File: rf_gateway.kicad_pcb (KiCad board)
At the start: 2 copper layers, 48.2 x 23.3 mm, 7 parts, among them J101 PJ-202A, J102 Conn_01x03_Female, J103 Conn_01x05_Male, U101 ESP32-WROOM-32

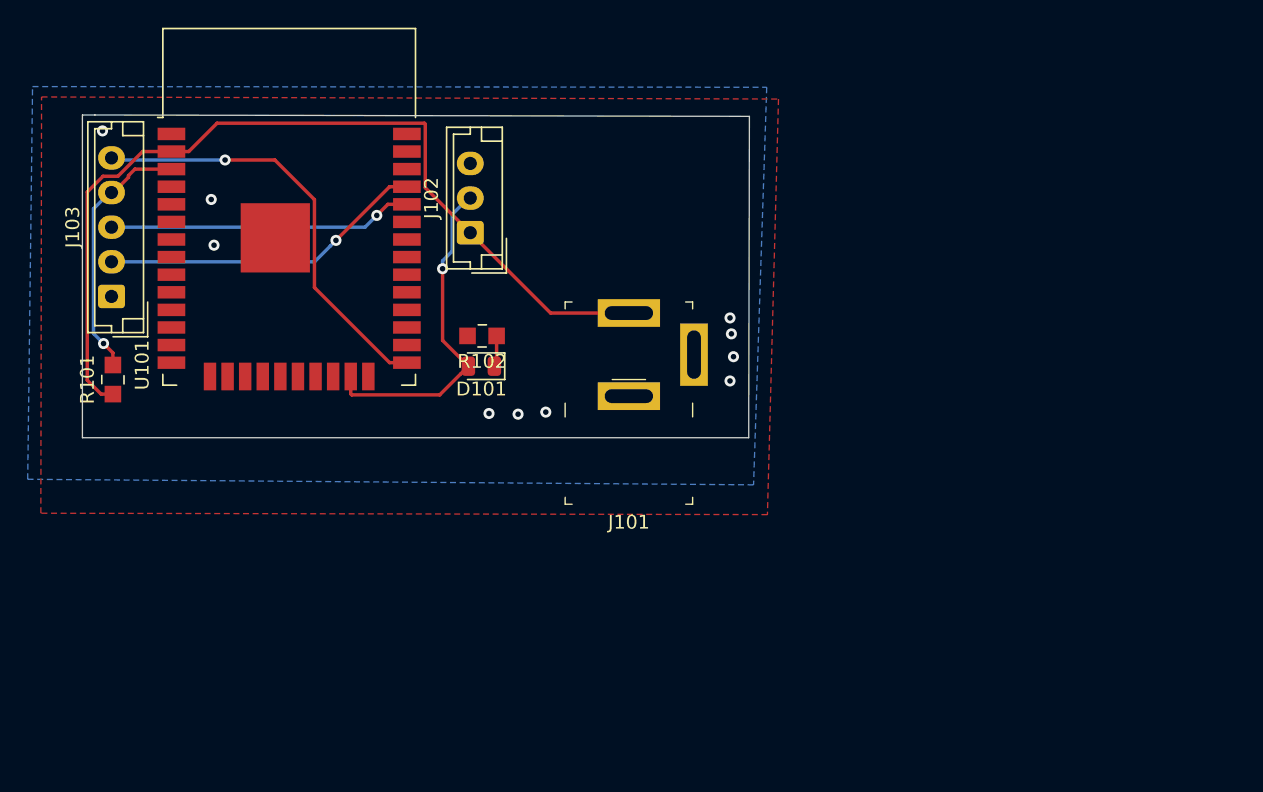
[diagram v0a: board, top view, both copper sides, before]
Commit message: First RC
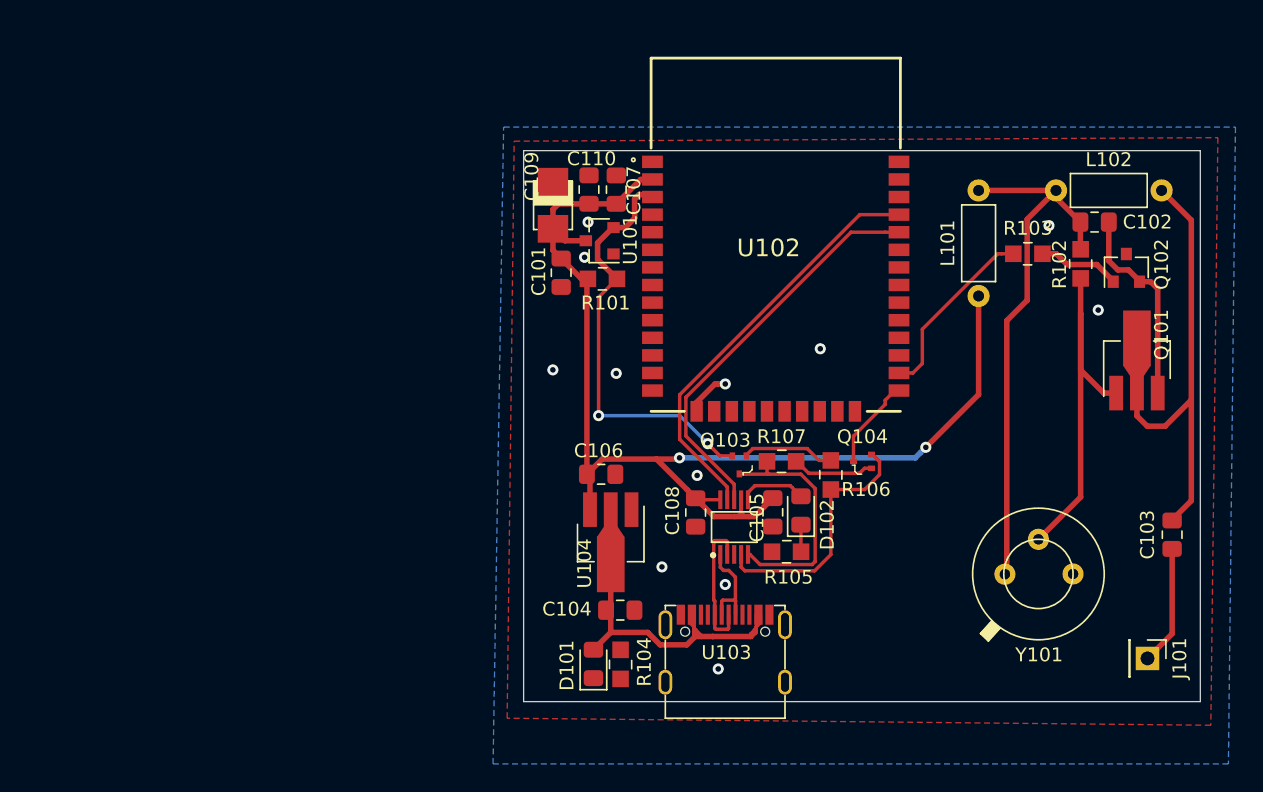
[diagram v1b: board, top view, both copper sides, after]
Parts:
- removed J102: Conn_01x03_Female, Connector_JST:JST_EH_B3B-EH-A_1x03_P2.50mm_Vertical
- removed J103: Conn_01x05_Male, Connector_JST:JST_EH_B5B-EH-A_1x05_P2.50mm_Vertical
- added C101: 100nF, Capacitor_SMD:C_0805_2012Metric_Pad1.15x1.40mm_HandSolder, F.Cu at (96.6, 66.1)
- added C102: 7pF, Capacitor_SMD:C_0805_2012Metric_Pad1.15x1.40mm_HandSolder, F.Cu at (135.1, 62.5)
- added C103: 7pF, Capacitor_SMD:C_0805_2012Metric_Pad1.15x1.40mm_HandSolder, F.Cu at (140.7, 85.0)
- added C104: 10uF, Capacitor_SMD:C_0805_2012Metric_Pad1.15x1.40mm_HandSolder, F.Cu at (100.9, 90.5)
- added C105: 100nF, Capacitor_SMD:C_0805_2012Metric_Pad1.15x1.40mm_HandSolder, F.Cu at (111.9, 83.4)
- added C106: 10uF, Capacitor_SMD:C_0805_2012Metric_Pad1.15x1.40mm_HandSolder, F.Cu at (99.5, 80.7)
- added C107: 100nF, Capacitor_SMD:C_0805_2012Metric_Pad1.15x1.40mm_HandSolder, F.Cu at (100.6, 60.1)
- added C108: 100nF, Capacitor_SMD:C_0805_2012Metric_Pad1.15x1.40mm_HandSolder, F.Cu at (106.3, 83.4)
- added C109: 100uF, custom-lib:TAJB107M010RNJ, F.Cu at (96.0, 61.3)
- added C110: 10uF, Capacitor_SMD:C_0805_2012Metric_Pad1.15x1.40mm_HandSolder, F.Cu at (98.6, 60.1)
- added D102: BLUE, LED_SMD:LED_0805_2012Metric_Pad1.15x1.40mm_HandSolder, F.Cu at (113.9, 83.3)
- added L101: 8 Turns, Inductor_THT:L_Axial_L5.3mm_D2.2mm_P7.62mm_Horizontal_Vishay_IM-1, F.Cu at (126.7, 67.8)
- added L102: 3 Turns, Inductor_THT:L_Axial_L5.3mm_D2.2mm_P7.62mm_Horizontal_Vishay_IM-1, F.Cu at (132.3, 60.2)
- added Q101: 2SC3357-T1-A, Package_TO_SOT_SMD:SOT-89-3_Handsoldering, F.Cu at (138.2, 72.8)
- added Q102: S8050, Package_TO_SOT_SMD:SOT-23, F.Cu at (137.4, 65.8)
- added Q103: Q_NPN_BCE, custom-lib:SOT-523, F.Cu at (109.5, 80.0)
- added Q104: Q_NPN_BCE, custom-lib:SOT-523, F.Cu at (118.4, 79.8)
- added R103: 27k, digikey-footprints:0805, F.Cu at (130.3, 64.8)
- added R104: 1k, digikey-footprints:0805, F.Cu at (100.9, 94.4)
- added R105: 1k, digikey-footprints:0805, F.Cu at (112.9, 86.3)
- added R106: 10k, digikey-footprints:0805, F.Cu at (116.1, 80.7)
- added R107: 10k, digikey-footprints:0805, F.Cu at (112.5, 79.8)
- added U102: ESP-32s, custom-lib:ESP-32S, F.Cu at (112.1, 76.1)
- added U103: C167321, custom-lib:C167321, F.Cu at (108.5, 91.5)
- added U104: HT7333-A, Package_TO_SOT_SMD:SOT-89-3_Handsoldering, F.Cu at (100.2, 85.2)
- added U105: CH340E, custom-lib:CH340E-MSOP-10, F.Cu at (109.1, 84.5)
- added Y101: 433MHz, custom-lib:C2280, F.Cu at (131.1, 87.9)
- D101: value LED -> RED; footprint Diode_SMD:D_0805_2012Metric -> LED_SMD:LED_0805_2012Metric_Pad1.15x1.40mm_HandSolder
- J101: value PJ-202A -> Antena; footprint digikey-footprints:Barrel_Jack_5.5mmODx2.1mmID_PJ-202A -> Connector_PinHeader_2.54mm:PinHeader_1x01_P2.54mm_Vertical
- R102: value 500 -> 27k
- U101: value ESP32-WROOM-32 -> TPS3839; footprint RF_Module:ESP32-WROOM-32 -> Package_TO_SOT_SMD:SOT-23
- moved R102 43.5 mm to (134.1, 65.5), turned to 90 degrees
- moved J101 43.4 mm to (138.9, 94.0), turned to 270 degrees
- moved R101 36.1 mm to (99.6, 66.6), turned to 180 degrees
- moved D101 23.0 mm to (98.9, 94.4), turned to 90 degrees
- moved U101 22.4 mm to (99.4, 63.8), turned to 180 degrees
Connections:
- D101 pad 2: Net-(D101-Pad2) -> +5V
- J101 pad 1: +3V3 -> Net-(C103-Pad2)
- R101 pad 1: +3V3 -> /EN
- R101 pad 2: /EN -> +3V3
- R102 pad 1: Net-(D101-Pad1) -> Net-(Q101-Pad1)
- R102 pad 2: GND -> Net-(C102-Pad1)
- U101 pad 2: +3V3 -> /EN
- U101 pad 3: /EN -> +3V3
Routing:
- net Net-(C102-Pad1): track 0.00 -> 39.9 mm
- net Net-(C103-Pad1): track 0.00 -> 36.0 mm
- net +5V: track 0.00 -> 29.1 mm
- net Net-(Q101-Pad1): track 0.00 -> 27.4 mm
- net /IO0: track 31.2 -> 6.65 mm, vias 1 -> 0
- net Net-(D101-Pad2): track 24.4 -> 0.00 mm, vias 1 -> 0
- net +3V3: track 65.4 -> 87.3 mm, vias 0 -> 2
- net /~RTS: track 0.00 -> 18.4 mm
- net /~CTS: track 0.00 -> 17.4 mm
- net Net-(C102-Pad2): track 0.00 -> 14.7 mm
- net /RF: track 0.00 -> 13.3 mm
- net /EN: track 18.7 -> 30.8 mm, vias 1 -> 2
- net /D-: track 0.00 -> 10.3 mm
- net Net-(C103-Pad2): track 0.00 -> 8.64 mm
- net /RX: track 22.0 -> 30.2 mm, vias 1 -> 0
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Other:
- board size 48.2 x 23.3 mm -> 48.8 x 39.8 mm
